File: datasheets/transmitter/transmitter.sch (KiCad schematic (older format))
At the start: 6 parts, among them CON1 AVR-ISP-6, IC1 ATTINY85-P, Q1 Q_NPN_EBC

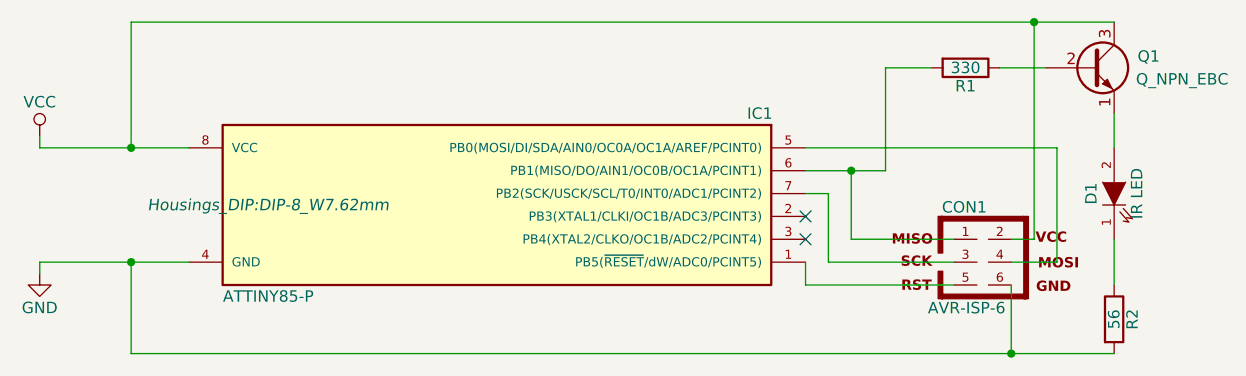
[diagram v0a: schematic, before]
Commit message: Revert "Kicad PCB layout"
This reverts commit 9afb40ae9a6d2ea0d6b4d8b9758429dc2c52fee4.
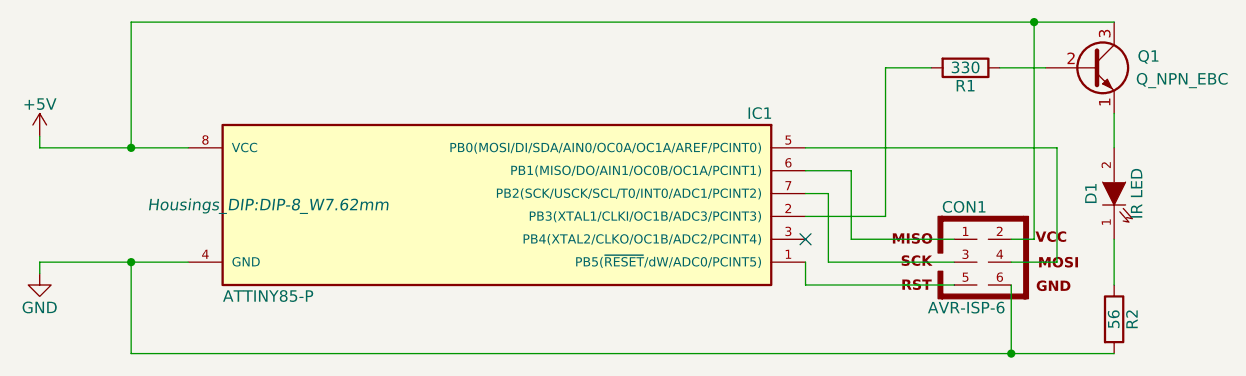
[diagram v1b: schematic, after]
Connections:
- net at IC1.2 (PB3(XTAL1/CLKI/OC1B/ADC3/PCINT3)): now also R1.2
- net at CON1.1, IC1.6 (PB1(MISO/DO/AIN1/OC0B/OC1A/PCINT1)): no longer R1.2
- net VCC renamed +5V
- no-connect marks 2 -> 1
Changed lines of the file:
@@
 LIBS:contrib
 LIBS:valves
-LIBS:transmitter-cache
 EELAYER 25 0
 EELAYER END
@@
 F 3 "" H 4000 4050 50  0000 C CNN
 	1    4000 4050
+	1    0    0    -1
+$EndComp
+$Comp
+L +5V #PWR02
+U 1 1 56C0E1BD
+P 4000 3450
+F 0 "#PWR02" H 4000 3300 50  0001 C CNN
+F 1 "+5V" H 4000 3590 50  0000 C CNN
+F 2 "" H 4000 3450 50  0000 C CNN
+F 3 "" H 4000 3450 50  0000 C CNN
+	1    4000 3450
 	1    0    0    -1
 $EndComp
@@
 	4400 4400 4400 4000
 Connection ~ 4400 4000
+Wire Wire Line
+	7700 3150 7700 3800
+Wire Wire Line
+	7700 3800 7350 3800
 $Comp
 L AVR-ISP-6 CON1
@@
 	7550 3900 7550 3600
 Wire Wire Line
-	7350 3600 7700 3600
+	7550 3600 7350 3600
 Wire Wire Line
 	8000 4000 7450 4000
@@
 Connection ~ 8250 4400
 NoConn ~ 7350 3900
-Wire Wire Line
-	7700 3600 7700 3150
-Connection ~ 7550 3600
-$Comp
-L VCC #PWR?
-U 1 1 56C27B48
-P 4000 3450
-F 0 "#PWR?" H 4000 3300 50  0001 C CNN
-F 1 "VCC" H 4000 3600 50  0000 C CNN
-F 2 "" H 4000 3450 50  0000 C CNN
-F 3 "" H 4000 3450 50  0000 C CNN
-	1    4000 3450
-	1    0    0    -1
-$EndComp
-NoConn ~ 7350 3800
 $EndSCHEMATC

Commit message: Kicad PCB layout
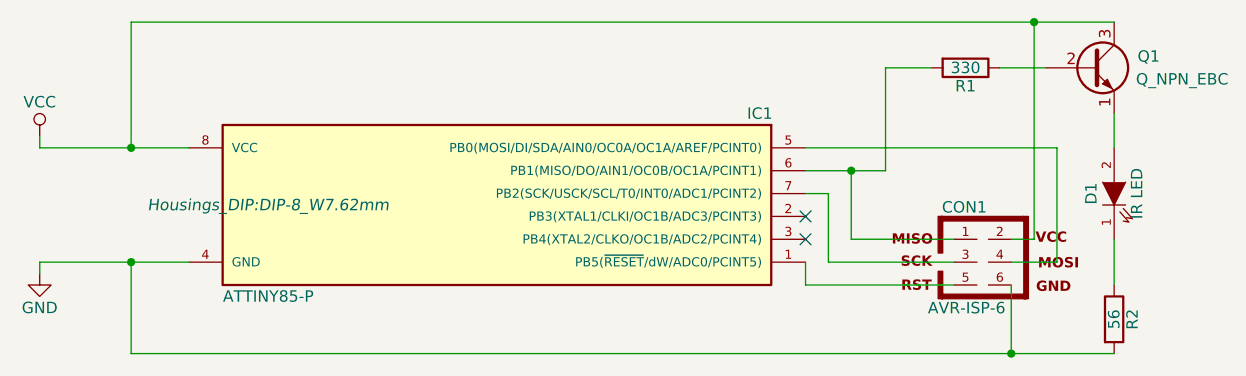
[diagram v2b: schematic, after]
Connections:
- net at IC1.2 (PB3(XTAL1/CLKI/OC1B/ADC3/PCINT3)): no longer R1.2
- net at CON1.1, IC1.6 (PB1(MISO/DO/AIN1/OC0B/OC1A/PCINT1)): now also R1.2
- net +5V renamed VCC
- no-connect marks 1 -> 2
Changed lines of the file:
@@
 LIBS:contrib
 LIBS:valves
+LIBS:transmitter-cache
 EELAYER 25 0
 EELAYER END
@@
 F 3 "" H 4000 4050 50  0000 C CNN
 	1    4000 4050
-	1    0    0    -1
-$EndComp
-$Comp
-L +5V #PWR02
-U 1 1 56C0E1BD
-P 4000 3450
-F 0 "#PWR02" H 4000 3300 50  0001 C CNN
-F 1 "+5V" H 4000 3590 50  0000 C CNN
-F 2 "" H 4000 3450 50  0000 C CNN
-F 3 "" H 4000 3450 50  0000 C CNN
-	1    4000 3450
 	1    0    0    -1
 $EndComp
@@
 	4400 4400 4400 4000
 Connection ~ 4400 4000
-Wire Wire Line
-	7700 3150 7700 3800
-Wire Wire Line
-	7700 3800 7350 3800
 $Comp
 L AVR-ISP-6 CON1
@@
 	7550 3900 7550 3600
 Wire Wire Line
-	7550 3600 7350 3600
+	7350 3600 7700 3600
 Wire Wire Line
 	8000 4000 7450 4000
@@
 Connection ~ 8250 4400
 NoConn ~ 7350 3900
+Wire Wire Line
+	7700 3600 7700 3150
+Connection ~ 7550 3600
+$Comp
+L VCC #PWR?
+U 1 1 56C27B48
+P 4000 3450
+F 0 "#PWR?" H 4000 3300 50  0001 C CNN
+F 1 "VCC" H 4000 3600 50  0000 C CNN
+F 2 "" H 4000 3450 50  0000 C CNN
+F 3 "" H 4000 3450 50  0000 C CNN
+	1    4000 3450
+	1    0    0    -1
+$EndComp
+NoConn ~ 7350 3800
 $EndSCHEMATC
